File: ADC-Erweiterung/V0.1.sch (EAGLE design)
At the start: 28 parts, among them IC1 ADS124S06IPBS, X1 33PIN-2.54, X2 MKDSN1,5/3-5,08, X3 A97581-ND, X4 A97581-ND, X5 A97581-ND, X6 MOLEX-8738-0343

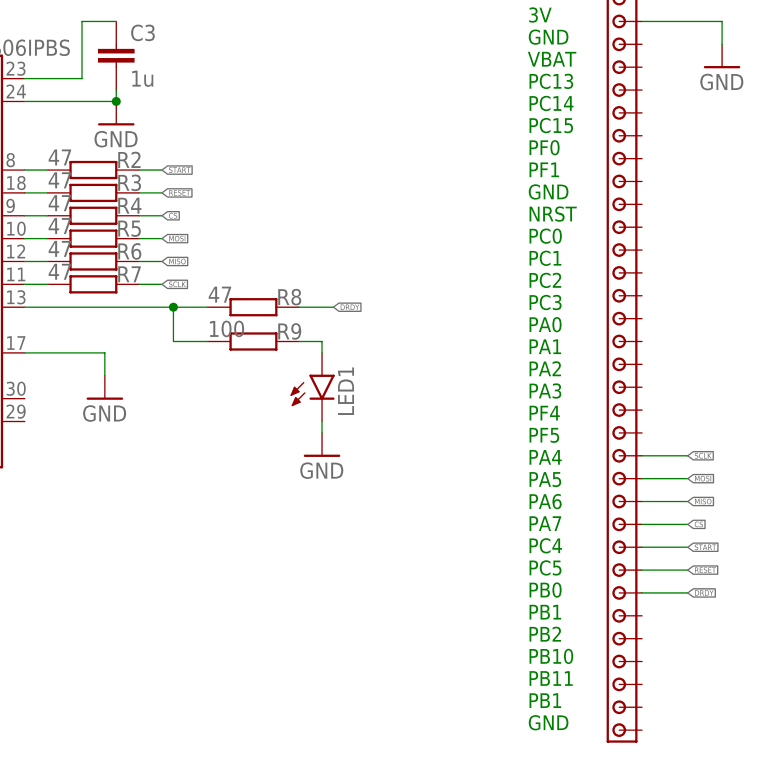
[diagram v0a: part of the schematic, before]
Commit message: Stand der Abgabe
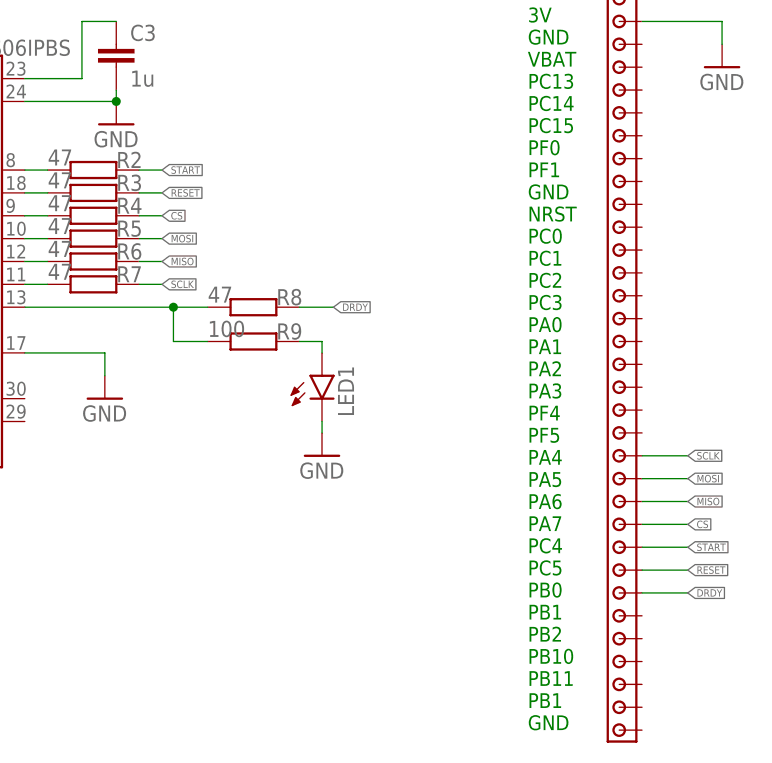
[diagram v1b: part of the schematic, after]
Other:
- note added: "PT100"
- note removed: "TP100"
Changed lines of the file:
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@@
 <?xml version="1.0" encoding="utf-8"?>
 <!DOCTYPE eagle SYSTEM "eagle.dtd">
-<eagle version="9.3.0">
+<eagle version="9.2.1">
 <drawing>
 <settings>
@@
 <setting verticaltext="up"/>
 </settings>
-<grid distance="1.27" unitdist="mm" unit="mm" style="lines" multiple="1" display="no" altdistance="0.01" altunitdist="inch" altunit="inch"/>
+<grid distance="0.1" unitdist="inch" unit="inch" style="lines" multiple="1" display="no" altdistance="0.01" altunitdist="inch" altunit="inch"/>
 <layers>
 <layer number="1" name="Top" color="4" fill="1" visible="no" active="no"/>
@@
 <wire x1="19.05" y1="77.47" x2="19.05" y2="92.71" width="0.1524" layer="90"/>
 <wire x1="19.05" y1="92.71" x2="-3.81" y2="92.71" width="0.1524" layer="90"/>
-<text x="-3.81" y="92.71" size="1.6764" layer="90">TP100</text>
+<text x="-3.81" y="92.71" size="1.6764" layer="90">PT100</text>
 </plain>
 <instances>
@@
 <pinref part="X1" gate="G$1" pin="21"/>
 <wire x1="196.85" y1="48.26" x2="201.93" y2="48.26" width="0.1524" layer="91"/>
-<label x="201.93" y="48.26" size="0.6096" layer="95" xref="yes"/>
-</segment>
-<segment>
-<label x="143.51" y="67.31" size="0.6096" layer="95" xref="yes"/>
+<label x="201.93" y="48.26" size="0.8128" layer="95" xref="yes"/>
+</segment>
+<segment>
+<label x="143.51" y="67.31" size="0.8128" layer="95" xref="yes"/>
 <pinref part="R7" gate="G$1" pin="2"/>
 <wire x1="140.97" y1="67.31" x2="143.51" y2="67.31" width="0.1524" layer="91"/>
@@
 <net name="MOSI" class="0">
 <segment>
-<label x="143.51" y="72.39" size="0.6096" layer="95" xref="yes"/>
+<label x="143.51" y="72.39" size="0.8128" layer="95" xref="yes"/>
 <pinref part="R5" gate="G$1" pin="2"/>
 <wire x1="140.97" y1="72.39" x2="143.51" y2="72.39" width="0.1524" layer="91"/>
@@
 <pinref part="X1" gate="G$1" pin="22"/>
 <wire x1="196.85" y1="45.72" x2="201.93" y2="45.72" width="0.1524" layer="91"/>
-<label x="201.93" y="45.72" size="0.6096" layer="95" xref="yes"/>
+<label x="201.93" y="45.72" size="0.8128" layer="95" xref="yes"/>
 </segment>
 </net>
@@
 <pinref part="X1" gate="G$1" pin="23"/>
 <wire x1="196.85" y1="43.18" x2="201.93" y2="43.18" width="0.1524" layer="91"/>
-<label x="201.93" y="43.18" size="0.6096" layer="95" xref="yes"/>
-</segment>
-<segment>
-<label x="143.51" y="69.85" size="0.6096" layer="95" xref="yes"/>
+<label x="201.93" y="43.18" size="0.8128" layer="95" xref="yes"/>
+</segment>
+<segment>
+<label x="143.51" y="69.85" size="0.8128" layer="95" xref="yes"/>
 <pinref part="R6" gate="G$1" pin="2"/>
 <wire x1="140.97" y1="69.85" x2="143.51" y2="69.85" width="0.1524" layer="91"/>
@@
 <net name="START" class="0">
 <segment>
-<label x="143.51" y="80.01" size="0.6096" layer="95" xref="yes"/>
+<label x="143.51" y="80.01" size="0.8128" layer="95" xref="yes"/>
 <pinref part="R2" gate="G$1" pin="2"/>
 <wire x1="140.97" y1="80.01" x2="143.51" y2="80.01" width="0.1524" layer="91"/>
@@
 <pinref part="X1" gate="G$1" pin="25"/>
 <wire x1="196.85" y1="38.1" x2="201.93" y2="38.1" width="0.1524" layer="91"/>
-<label x="201.93" y="38.1" size="0.6096" layer="95" xref="yes"/>
+<label x="201.93" y="38.1" size="0.8128" layer="95" xref="yes"/>
 </segment>
 </net>
@@
 <pinref part="X1" gate="G$1" pin="24"/>
 <wire x1="196.85" y1="40.64" x2="201.93" y2="40.64" width="0.1524" layer="91"/>
-<label x="201.93" y="40.64" size="0.6096" layer="95" xref="yes"/>
-</segment>
-<segment>
-<label x="143.51" y="74.93" size="0.6096" layer="95" xref="yes"/>
+<label x="201.93" y="40.64" size="0.8128" layer="95" xref="yes"/>
+</segment>
+<segment>
+<label x="143.51" y="74.93" size="0.8128" layer="95" xref="yes"/>
 <pinref part="R4" gate="G$1" pin="2"/>
 <wire x1="140.97" y1="74.93" x2="143.51" y2="74.93" width="0.1524" layer="91"/>
@@
 <pinref part="X1" gate="G$1" pin="26"/>
 <wire x1="196.85" y1="35.56" x2="201.93" y2="35.56" width="0.1524" layer="91"/>
-<label x="201.93" y="35.56" size="0.6096" layer="95" xref="yes"/>
-</segment>
-<segment>
-<label x="143.51" y="77.47" size="0.6096" layer="95" xref="yes"/>
+<label x="201.93" y="35.56" size="0.8128" layer="95" xref="yes"/>
+</segment>
+<segment>
+<label x="143.51" y="77.47" size="0.8128" layer="95" xref="yes"/>
 <pinref part="R3" gate="G$1" pin="2"/>
 <wire x1="140.97" y1="77.47" x2="143.51" y2="77.47" width="0.1524" layer="91"/>
@@
 <pinref part="X1" gate="G$1" pin="27"/>
 <wire x1="196.85" y1="33.02" x2="201.93" y2="33.02" width="0.1524" layer="91"/>
-<label x="201.93" y="33.02" size="0.6096" layer="95" xref="yes"/>
-</segment>
-<segment>
-<label x="162.56" y="64.77" size="0.6096" layer="95" xref="yes"/>
+<label x="201.93" y="33.02" size="0.8128" layer="95" xref="yes"/>
+</segment>
+<segment>
+<label x="162.56" y="64.77" size="0.8128" layer="95" xref="yes"/>
 <pinref part="R8" gate="G$1" pin="2"/>
 <wire x1="158.75" y1="64.77" x2="162.56" y2="64.77" width="0.1524" layer="91"/>
